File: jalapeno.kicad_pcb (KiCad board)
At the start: 2 copper layers, 233.4 x 81 mm, 133 parts, among them IC1 ATMEGA32U4-AU, J1 USB_B, J2 AVR-ISP-6, J3 Conn_01x04, K1 esc, K10 o, K11 p, K12 back, K13 tab, K14 a, K15 s, K16 d, K17 f, K18 g, K19 h, K2 q, K20 j, K21 k, K22 l, K23 ;, K24 caps, K25 caps, K26 z, K27 x, K28 c, K29 v, K3 w, K30 b, K31 n, K32 m, K33 ,, K33_1 ,, K34 ., K34_1 ., K35 ctrl, K36 gui, K37 alt, K37_1 alt, K38 space, K38_1 space, K39 alt, K39_1 gui, K4 e, K40 gui, K41 ctrl, K42 KEYSW, K5 r, K6 t, K7 y, K8 u, K9 i, SW1 SW_PUSH, U1 MDBT40, U2 SPX3819M5-L-3-3, U3 MCP73831T-2ACI/OT, Y1 XTAL_GND

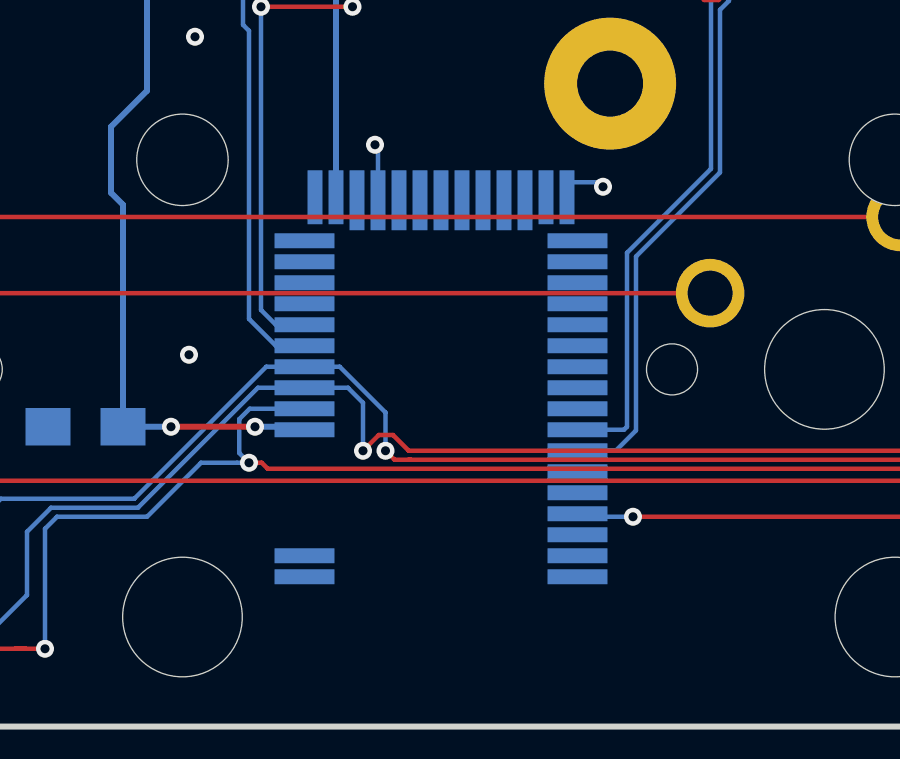
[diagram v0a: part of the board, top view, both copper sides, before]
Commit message: gerber export & logo
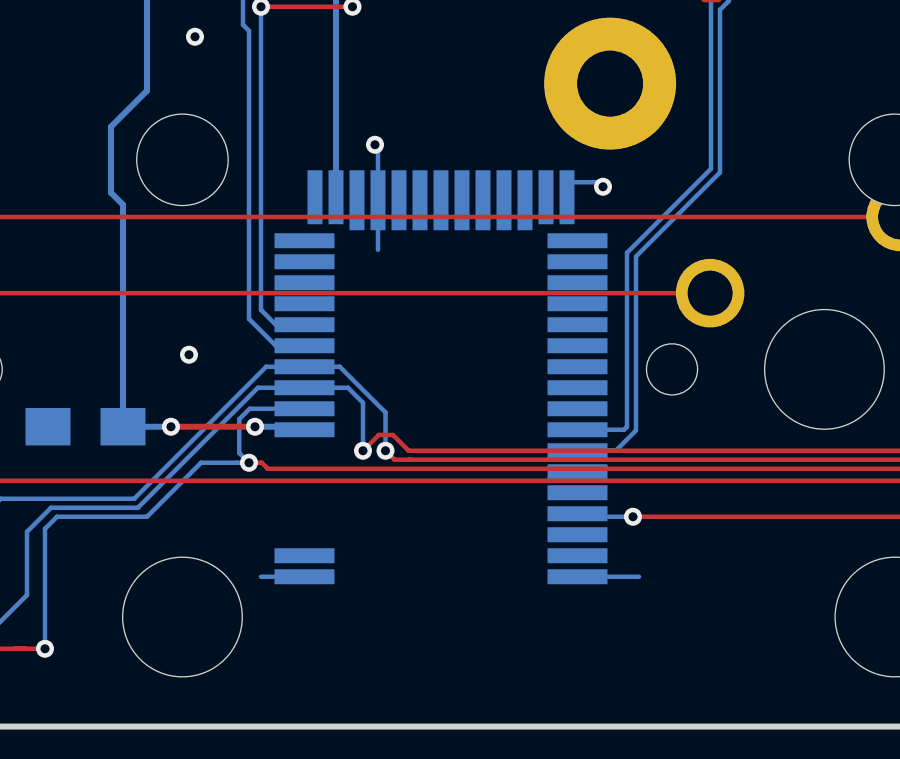
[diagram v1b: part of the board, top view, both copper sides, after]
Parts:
- added G***: LOGO, Jalapeno:LOGO_MASK, F.Cu at (73.6, 98.6)
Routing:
- net GND: track 33.3 -> 37.9 mm
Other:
- board text added: "BLE"
- board text added: "V0.0.2"
